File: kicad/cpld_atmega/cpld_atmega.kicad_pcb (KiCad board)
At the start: 2 copper layers, 106.7 x 58.4 mm, 33 parts, among them CON1 AVR-ISP-6, J1 PWR, J10 FB 4, J2 ADC, J3 Port B, J4 PORT D, J5 Port C, J6 FB 1, J7 FB 2, J8 JTAG, J9 FB 3, SW1 SW_Push, SW2 PWR, U1 LM1117-3.3, U2 ATMEGA168A-AU, U3 XC9572XL-VQFP44, Y1 12Mhz

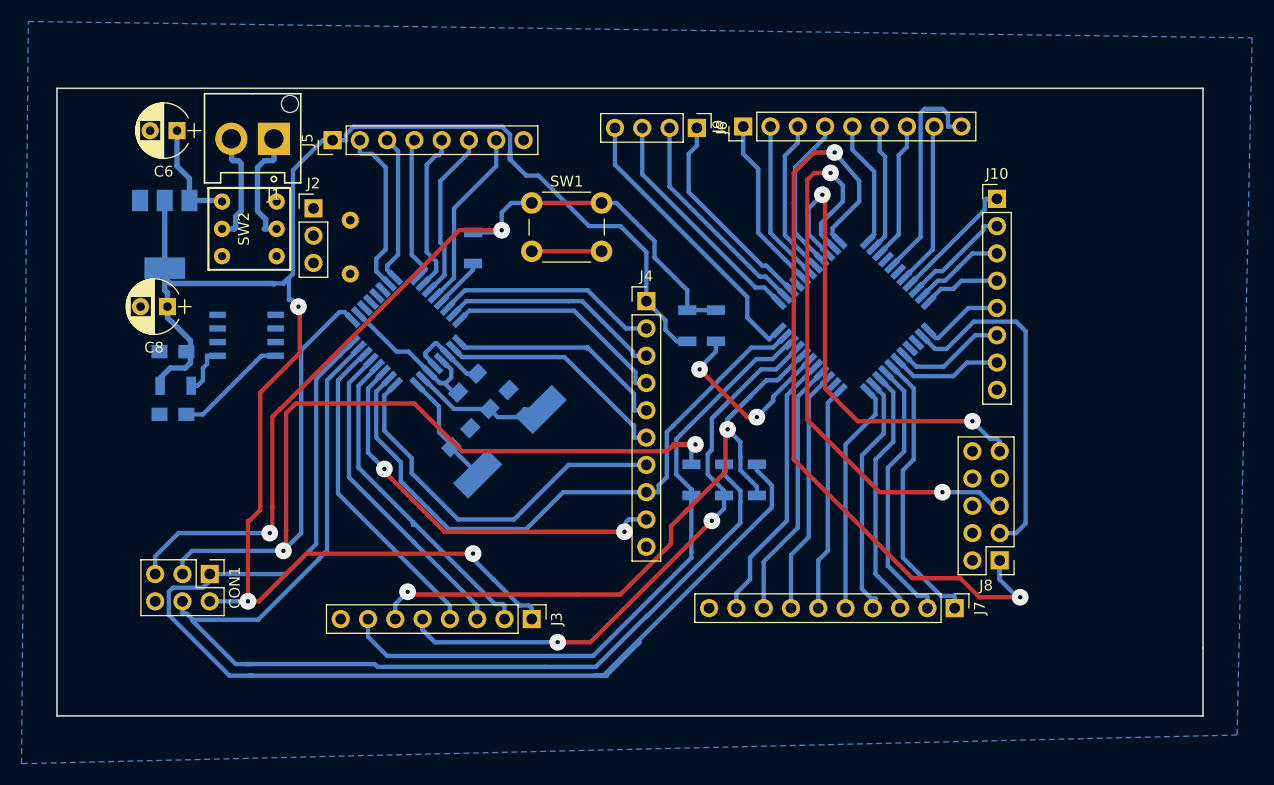
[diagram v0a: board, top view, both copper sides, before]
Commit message: 1.version almost done
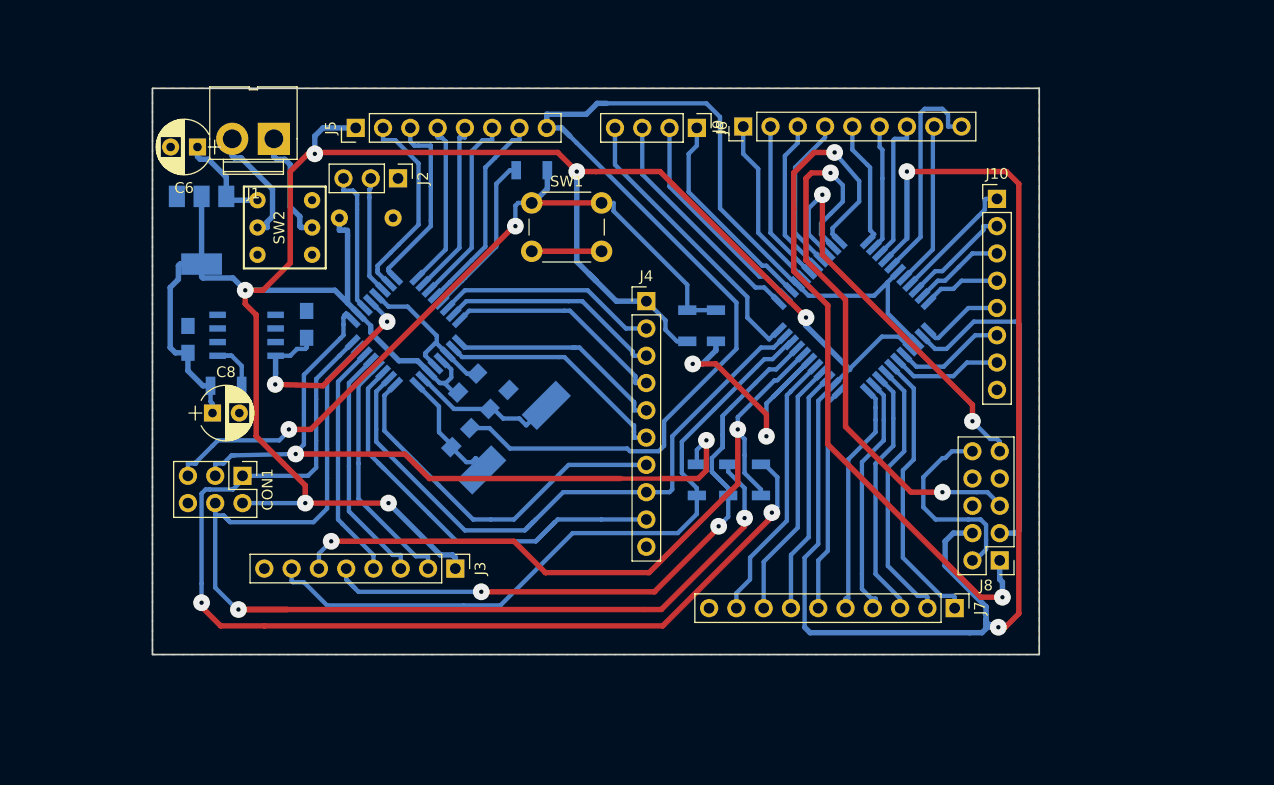
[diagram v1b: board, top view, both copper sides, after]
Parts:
- J1: footprint Connectors_Hirose:Hirose_DF63-2P-3.96DSA_02x3.96mm_Straight -> Connectors:JWT_Vertical_A3963-RM3.96mm-2
- moved C1 15.0 mm to (37.2, 66.4), turned to 90 degrees
- moved C8 10.8 mm to (28.4, 74.7), turned to 0 degrees
- moved CON1 9.64 mm to (31.2, 80.5)
- moved R3 9.07 mm to (58.2, 52.1), turned to 180 degrees
- moved J3 8.52 mm to (51.1, 89.2)
- moved J2 8.36 mm to (45.7, 52.8), turned to 270 degrees
- moved C5 5.31 mm to (40.3, 56.5), turned to 0 degrees
- moved R1 4.70 mm to (29.7, 72.1)
- moved U1 3.45 mm to (27.4, 57.7)
- moved SW2 3.30 mm to (35.2, 57.4)
- moved J5 2.44 mm to (41.8, 48.1)
- moved C6 2.44 mm to (27.1, 49.9)
- moved C9 1.81 mm to (26.2, 67.8), turned to 90 degrees
- moved Y1 0.54 mm to (56.5, 77.0)
- moved R6 0.51 mm to (73.5, 80.9)
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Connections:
- J8 pad 6: Net-(J8-Pad6) -> (no net)
- J8 pad 7: Net-(J8-Pad7) -> (no net)
- J8 pad 8: Net-(J8-Pad8) -> (no net)
- SW2 pad 1: (no net) -> Net-(SW2-Pad1)
- SW2 pad 6: (no net) -> Net-(SW2-Pad6)
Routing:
- net VCC: track 180.8 -> 352.4 mm, vias 3 -> 8
- net GND: track 15.1 -> 156.6 mm
- net +2V5: track 10.6 -> 30.6 mm, vias 0 -> 2
- net /SCK: track 94.9 -> 75.3 mm
- net Net-(J2-Pad3): track 0.00 -> 15.0 mm
- net Net-(R7-Pad1): track 17.7 -> 32.5 mm
- net /MISO: track 114.2 -> 99.8 mm, vias 0 -> 2
- net /RESET: track 84.2 -> 71.6 mm
- net Net-(J2-Pad2): track 0.00 -> 11.2 mm
- net Net-(R3-Pad2): track 4.79 -> 15.5 mm
- net /MOSI_: track 58.0 -> 66.3 mm
- net Net-(J3-Pad2): track 30.8 -> 22.9 mm
- net Net-(J3-Pad4): track 30.1 -> 22.5 mm
- net Net-(J3-Pad3): track 29.9 -> 22.7 mm
- net /TDI: track 44.1 -> 37.9 mm
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- added copper zone on F.Cu, net GND
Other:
- board size 106.7 x 58.4 mm -> 82.5 x 52.7 mm
